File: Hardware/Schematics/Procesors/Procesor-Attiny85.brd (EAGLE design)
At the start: 27.3 x 27.3 mm, 7 parts

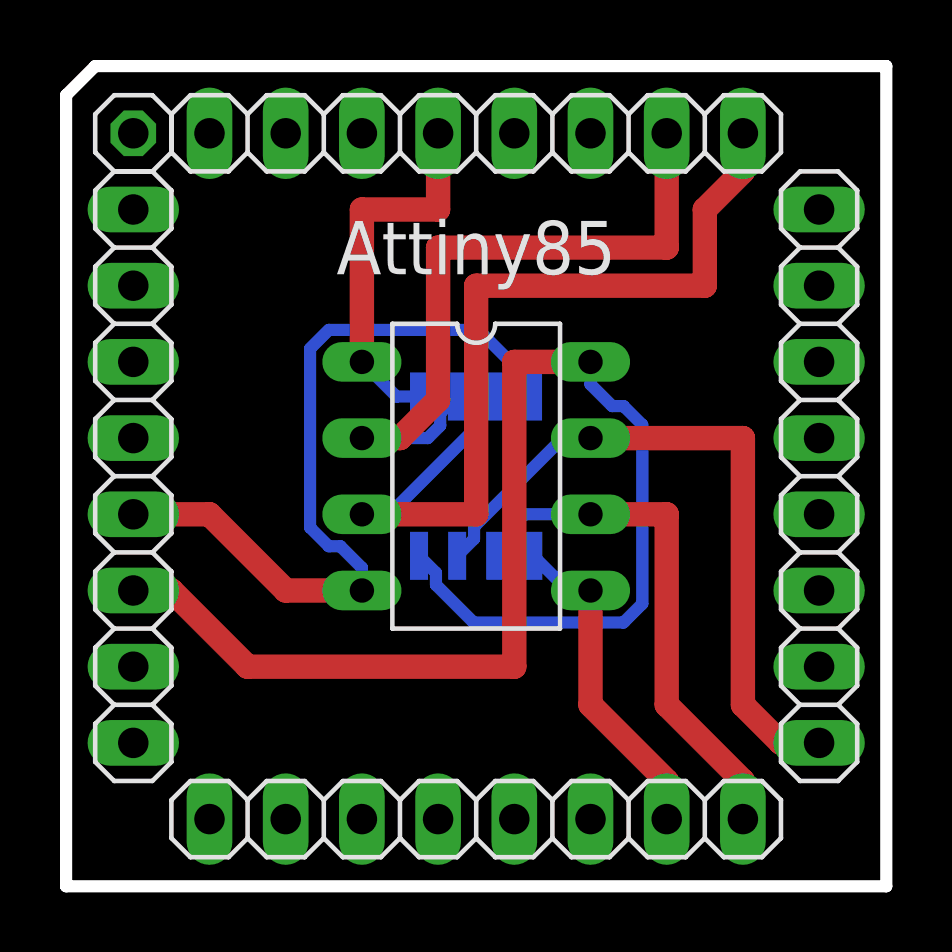
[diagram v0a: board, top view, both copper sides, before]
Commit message: commit
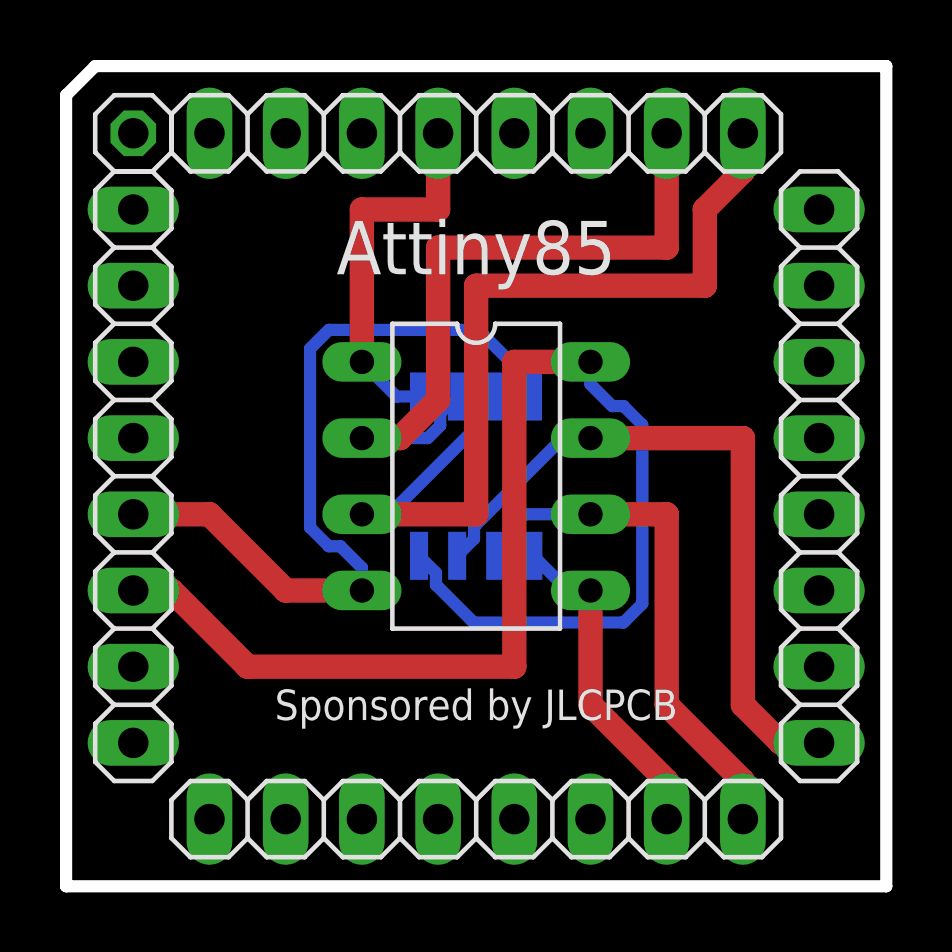
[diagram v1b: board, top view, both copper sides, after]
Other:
- board text added: "Sponsored by JLCPCB"
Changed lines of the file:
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@@
 <text x="0" y="7.62" size="1.778" layer="21" align="center">Attiny85</text>
 <text x="0" y="7.62" size="1.778" layer="22" rot="MR0" align="center">Attiny85</text>
+<text x="0" y="-7.62" size="1.016" layer="21" align="center">Sponsored by JLCPCB</text>
 </plain>
 <attributes>

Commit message: gerber update
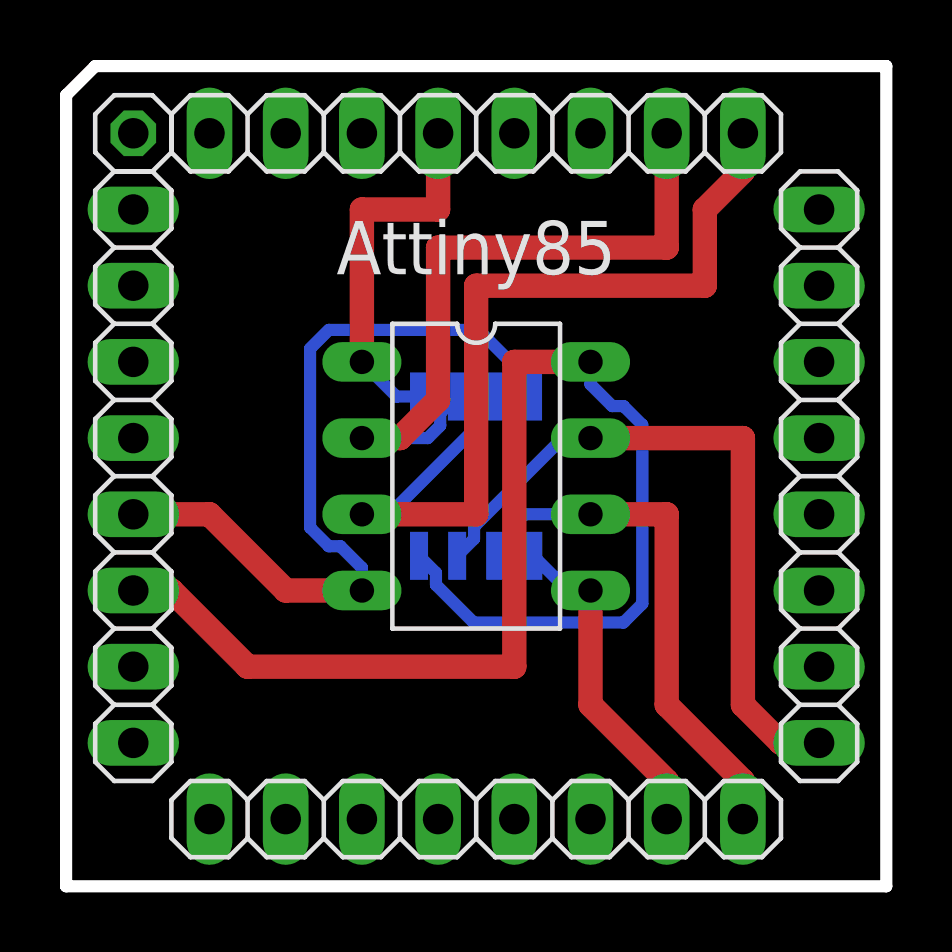
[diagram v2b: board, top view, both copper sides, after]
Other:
- board text removed: "Sponsored by JLCPCB"
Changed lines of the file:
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@@
 <?xml version="1.0" encoding="utf-8"?>
 <!DOCTYPE eagle SYSTEM "eagle.dtd">
-<eagle version="9.2.2">
+<eagle version="9.4.0">
 <drawing>
 <settings>
@@
 <text x="0" y="7.62" size="1.778" layer="21" align="center">Attiny85</text>
 <text x="0" y="7.62" size="1.778" layer="22" rot="MR0" align="center">Attiny85</text>
-<text x="0" y="-7.62" size="1.016" layer="21" align="center">Sponsored by JLCPCB</text>
 </plain>
 <attributes>
